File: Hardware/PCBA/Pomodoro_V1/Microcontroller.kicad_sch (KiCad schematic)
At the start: 7 parts, among them J1 Conn_01x10_Pin, J2 Conn_01x04_Pin, U1 STM32G071RBTx

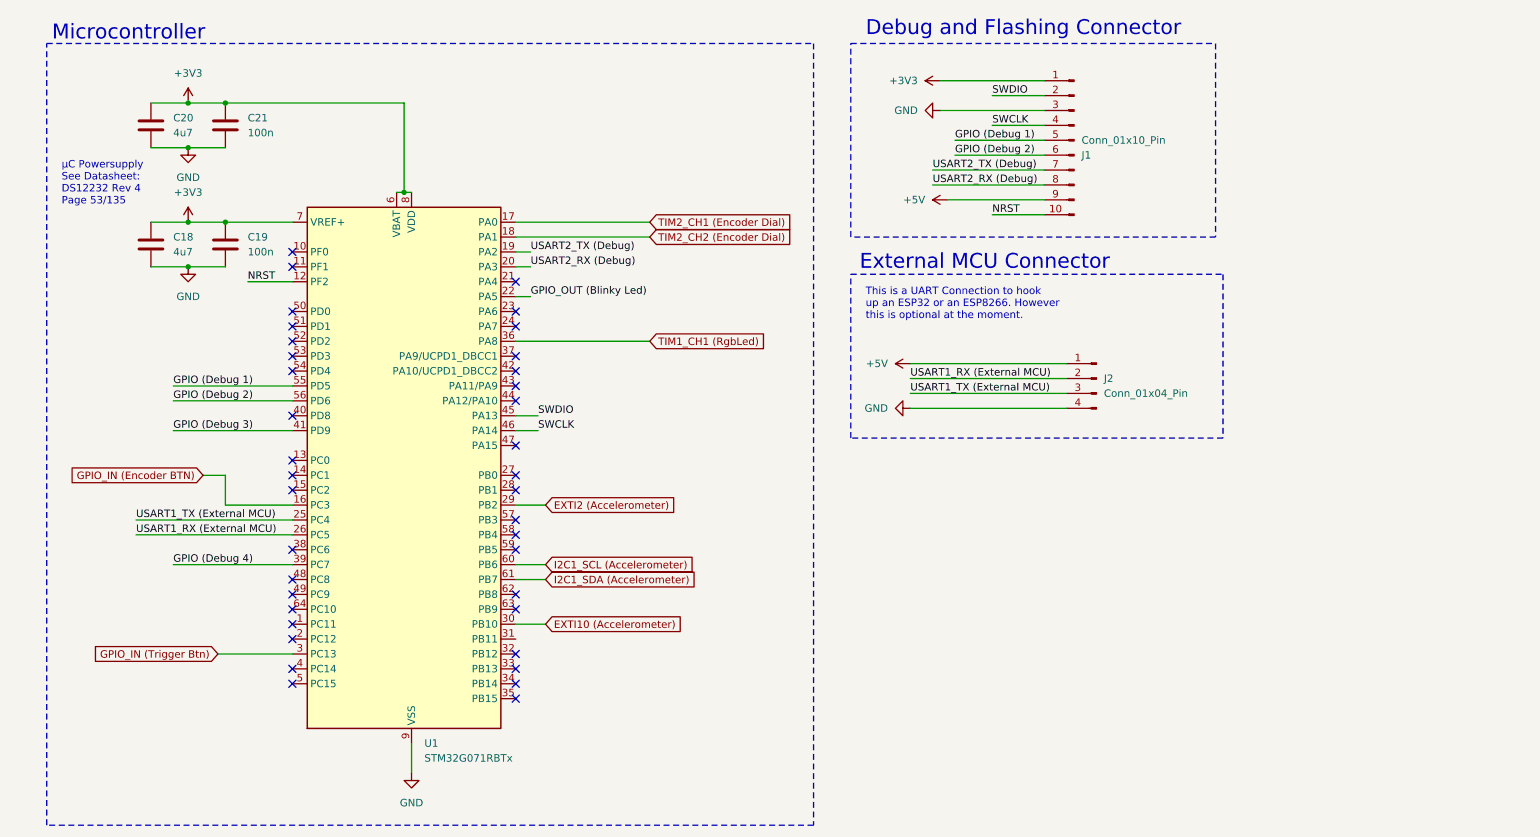
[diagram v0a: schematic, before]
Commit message: Finalized the schematic, First Draft of the finished Layout
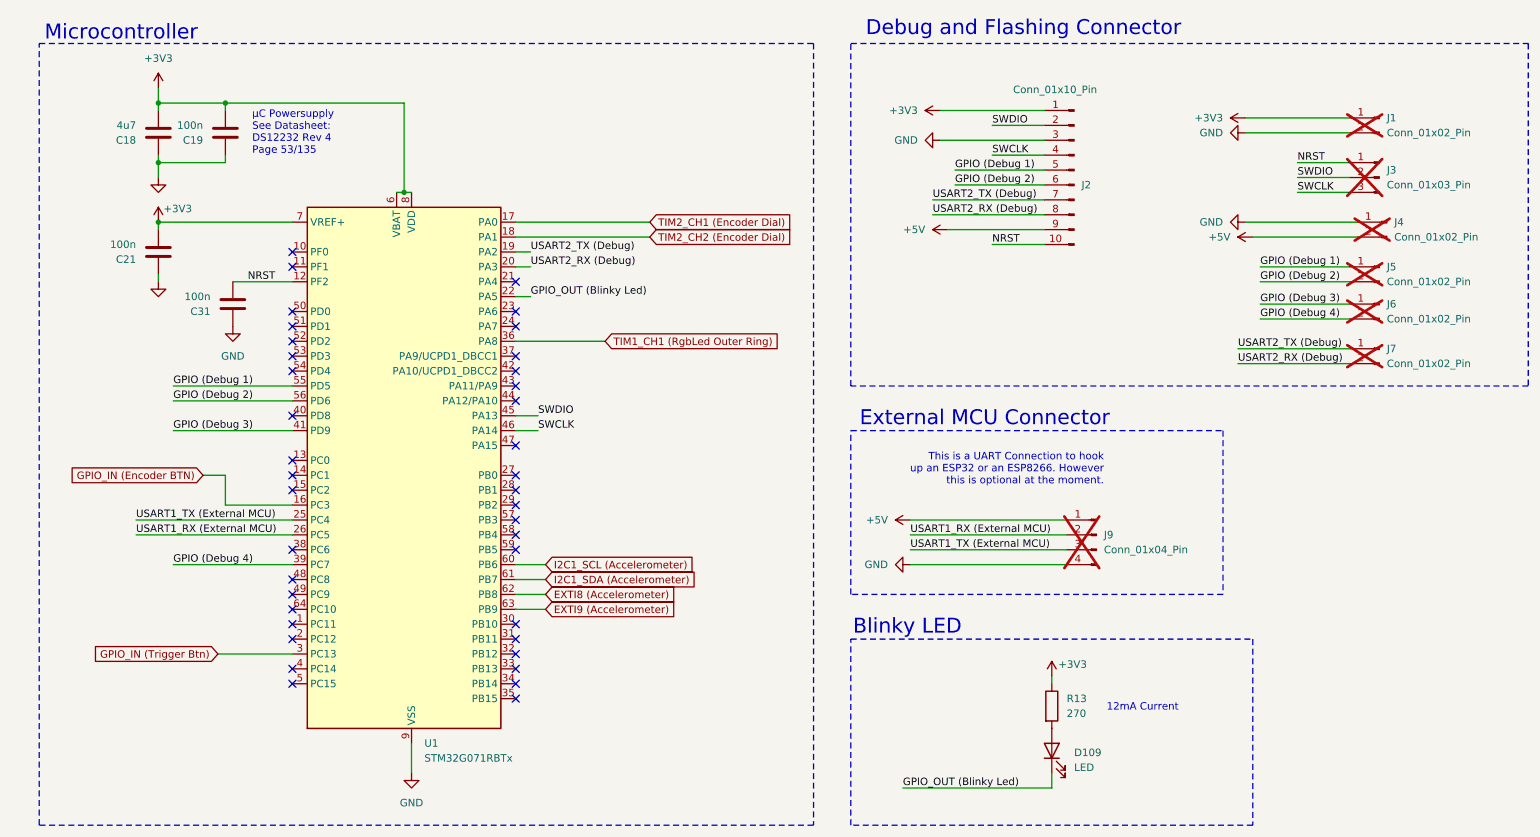
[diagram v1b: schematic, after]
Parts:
- removed C20: 4u7, symbol Device:C
- added C31: 100n, Capacitor_SMD:C_0805_2012Metric, symbol Device:C
- added D109: LED, Resistor_SMD:R_0603_1608Metric, symbol Device:LED
- added J1, J4, J5, J6, J7: Conn_01x02_Pin, Connector_PinHeader_2.54mm:PinHeader_1x02_P2.54mm_Vertical, symbol Connector:Conn_01x02_Pin
- added J3: Conn_01x03_Pin, Connector_PinHeader_2.54mm:PinHeader_1x03_P2.54mm_Vertical, symbol Connector:Conn_01x03_Pin
- added R13: 270, Resistor_SMD:R_0805_2012Metric, symbol Device:R
- C18, C19, C21: footprint (none) -> Capacitor_SMD:C_0805_2012Metric
- J2: renamed from J1; footprint (none) -> Connector:Tag-Connect_TC2050-IDC-NL_2x05_P1.27mm_Vertical
- J9: renamed from J2; footprint (none) -> Connector_PinHeader_2.54mm:PinHeader_1x04_P2.54mm_Vertical; now not fitted
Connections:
- net +3V3: now also C18.2, C19.2, C21.2, J1.1 (Pin_1), R13.1; no longer C18.1, C19.1, C21.1
- net +5V: now also J4.2 (Pin_2)
- net GND: now also C18.1, C19.1, C21.1, C31.1, J1.2 (Pin_2), J4.1 (Pin_1); no longer C18.2, C19.2, C21.2
- net GPIO (Debug 1): now also J5.1 (Pin_1)
- net GPIO (Debug 2): now also J5.2 (Pin_2)
- net GPIO (Debug 3): now also J6.1 (Pin_1)
- net GPIO (Debug 4): now also J6.2 (Pin_2)
- net GPIO_OUT (Blinky Led): now also D109.1 (K)
- net NRST: now also C31.2, J3.1 (Pin_1)
- net SWCLK: now also J3.3 (Pin_3)
- net SWDIO: now also J3.2 (Pin_2)
- net USART2_RX (Debug): now also J7.2 (Pin_2)
- net USART2_TX (Debug): now also J7.1 (Pin_1)
- net EXTI8 (Accelerometer): now reaches U1.62 (PB8)
- net EXTI9 (Accelerometer): now reaches U1.63 (PB9)
- net EXTI10 (Accelerometer): no longer names the net of U1.30 (PB10)
- net EXTI2 (Accelerometer): no longer names the net of U1.29 (PB2)
- net TIM1_CH1 (RgbLed) renamed TIM1_CH1 (RgbLed Outer Ring)
- new net: D109.2 (A), R13.2
- no-connect marks 38 -> 39
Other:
- note added: "12mA Current"
- note added: "Blinky LED"
- moved on the sheet: J2
